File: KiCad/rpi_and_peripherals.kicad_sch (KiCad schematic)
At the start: 5 parts, among them U4 PCM1808-Q1_PW_14, U9 PCM5102APW

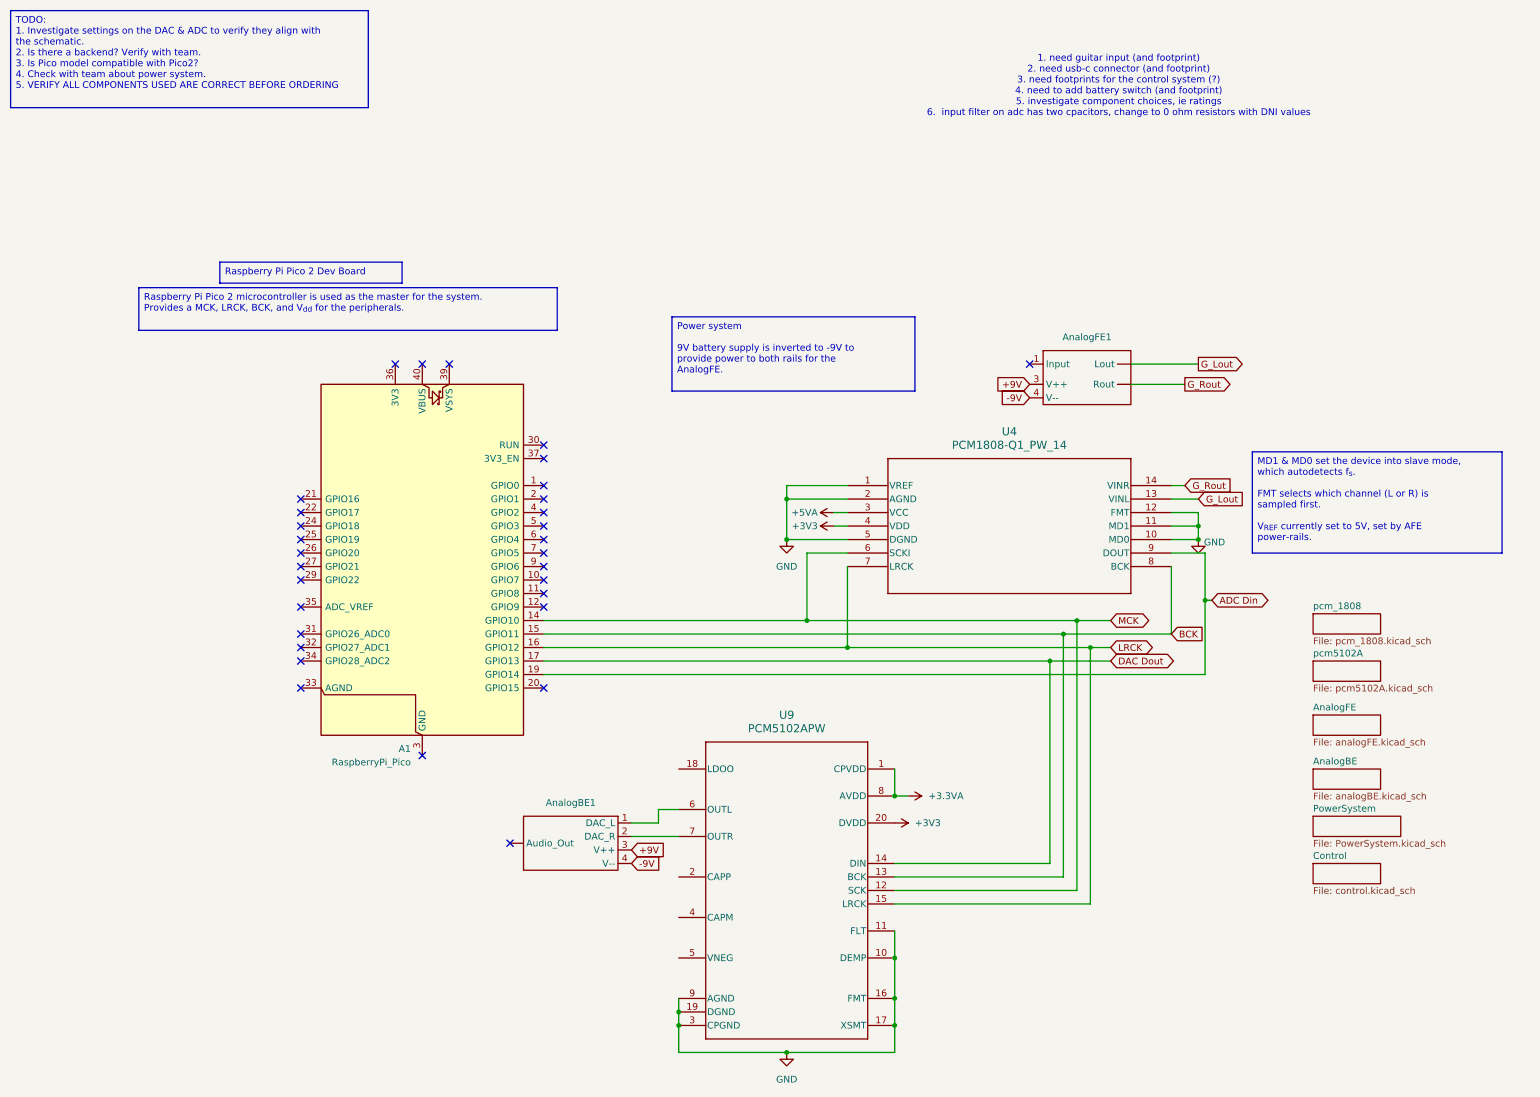
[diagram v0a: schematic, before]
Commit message: Best one yet
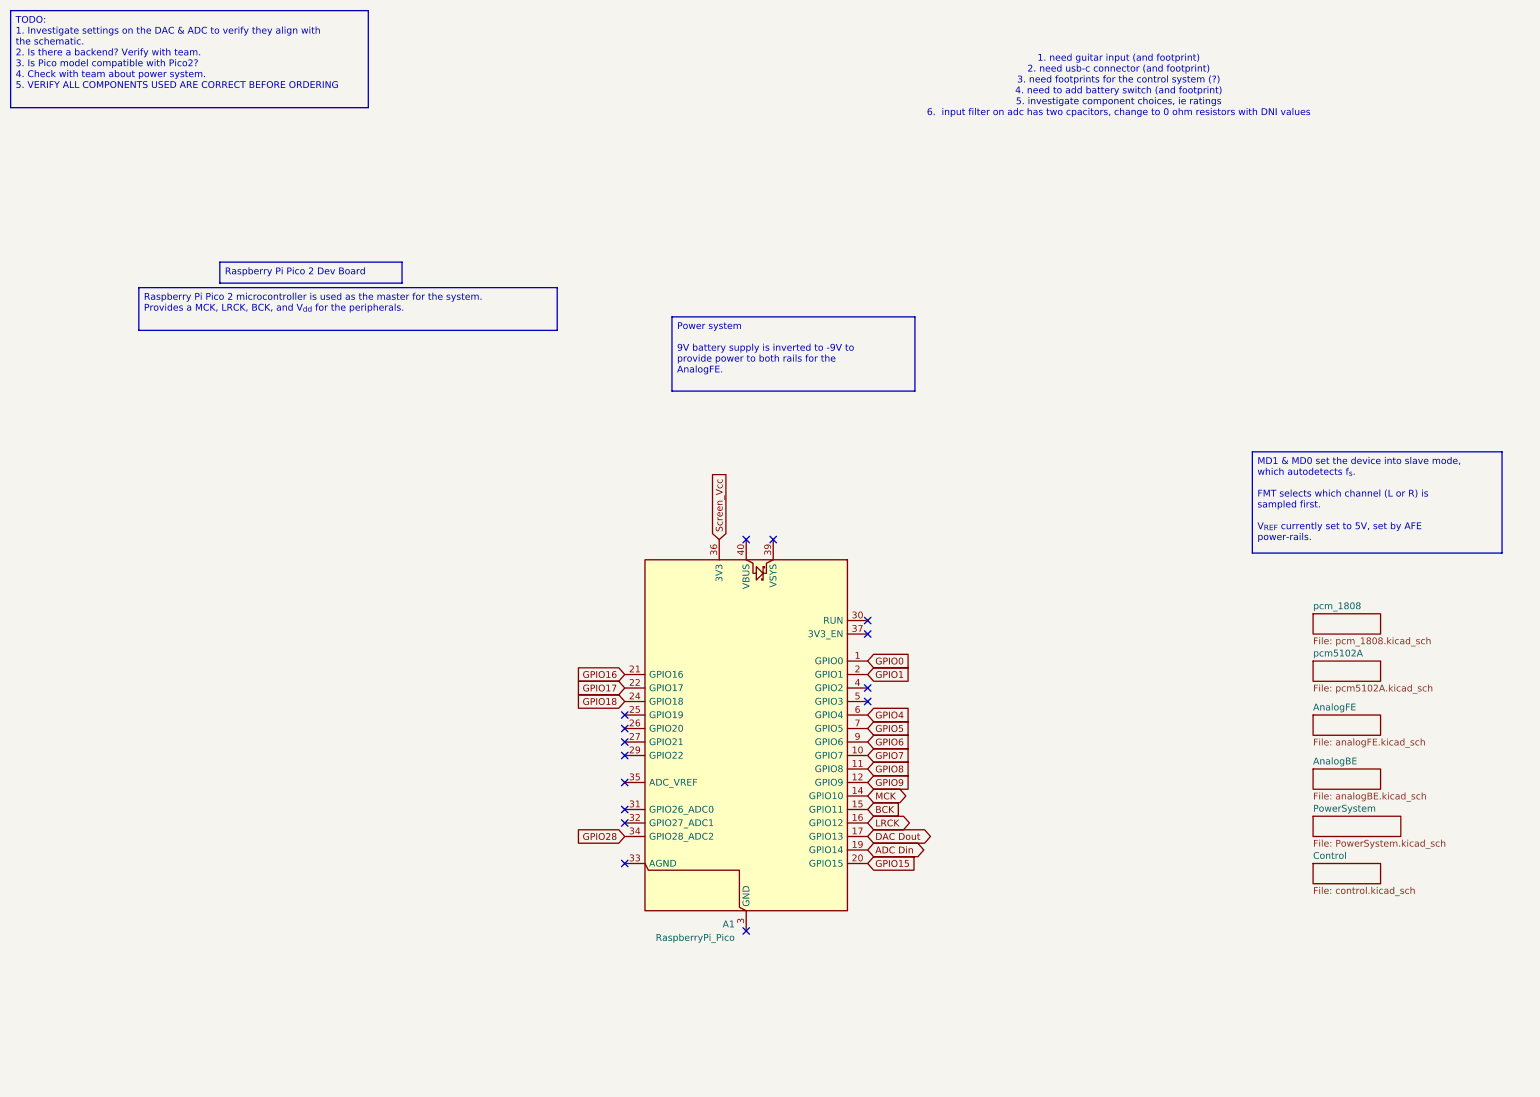
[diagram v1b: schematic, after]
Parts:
- removed AnalogBE1: (no value), symbol PCM1808:Analog_BE
- removed AnalogFE1: (no value), symbol PCM1808:Analoge_FE
- removed U4: PCM1808-Q1_PW_14, PW14_TEX, symbol PCM1808:PCM1808-Q1_PW_14
- removed U9: PCM5102APW, Package_SO:Texas_PW0020A_TSSOP-20_4.4x6.5mm_P0.65mm, symbol DAC:PCM5102APW
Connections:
- net GPIO0: now reaches A1.1 (GPIO0)
- net GPIO7: now reaches A1.10 (GPIO7)
- net GPIO8: now reaches A1.11 (GPIO8)
- net GPIO9: now reaches A1.12 (GPIO9)
- net GPIO1: now reaches A1.2 (GPIO1)
- net GPIO15: now reaches A1.20 (GPIO15)
- net GPIO16: now reaches A1.21 (GPIO16)
- net GPIO17: now reaches A1.22 (GPIO17)
- net GPIO18: now reaches A1.24 (GPIO18)
- net GPIO28: now reaches A1.34 (GPIO28_ADC2)
- net Screen_Vcc: now reaches A1.36 (3V3)
- net GPIO4: now reaches A1.6 (GPIO4)
- net GPIO5: now reaches A1.7 (GPIO5)
- net GPIO6: now reaches A1.9 (GPIO6)
- no-connect marks 31 -> 15
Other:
- moved on the sheet: A1
